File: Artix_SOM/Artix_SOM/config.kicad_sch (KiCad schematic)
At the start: 9 parts, among them SW1 SW_Push, U1 XC7A100T-FGG676

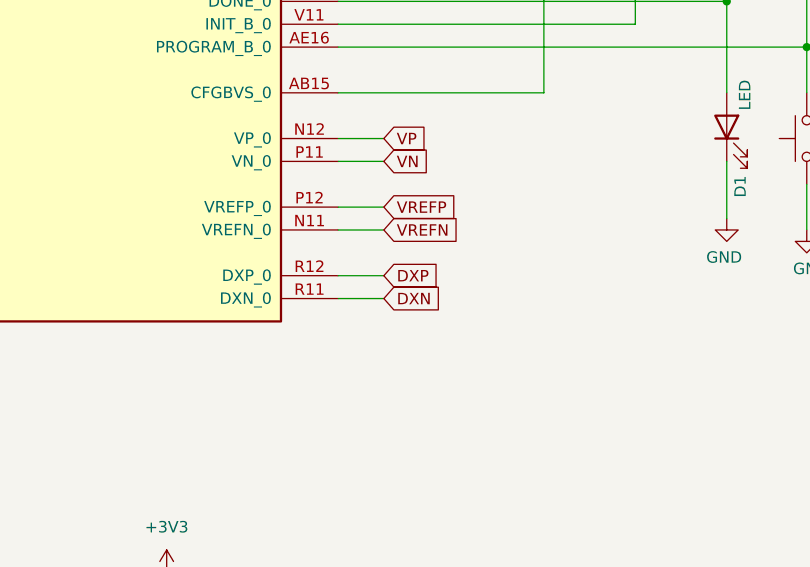
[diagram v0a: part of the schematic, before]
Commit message: update
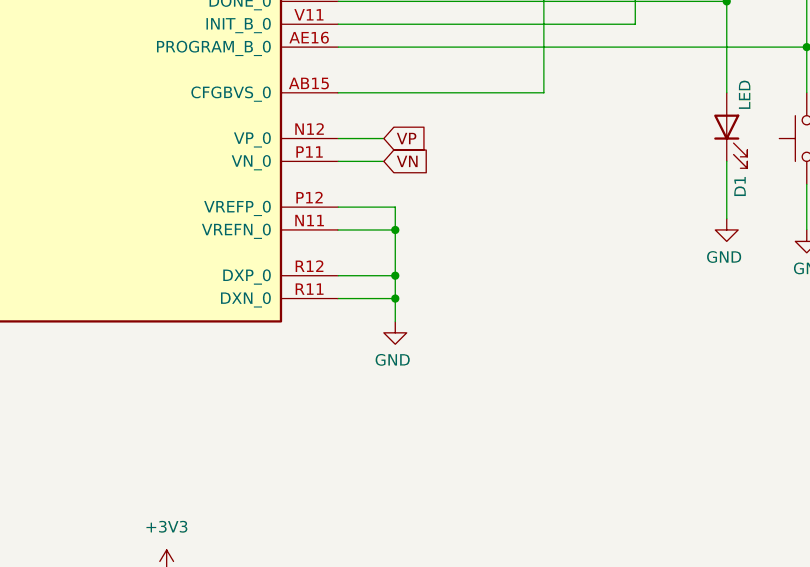
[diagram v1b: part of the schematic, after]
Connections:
- net DXN is gone; now on net GND: U1.R11 (DXN_0)
- net DXP is gone; now on net GND: U1.R12 (DXP_0)
- net VREFN is gone; now on net GND: U1.N11 (VREFN_0)
- net VREFP is gone; now on net GND: U1.P12 (VREFP_0)
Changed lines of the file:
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@@
+	)
+	(junction
+		(at 160.02 139.7)
+		(diameter 0)
+		(color 0 0 0 0)
+	)
+	(junction
+		(at 160.02 142.24)
+		(diameter 0)
+		(color 0 0 0 0)
 	)
 	(junction
@@
 	)
 	(junction
+		(at 160.02 134.62)
+		(diameter 0)
+		(color 0 0 0 0)
+	)
+	(junction
 		(at 191.77 93.98)
 		(diameter 0)
@@
 	(wire
 		(pts
+			(xy 160.02 132.08) (xy 160.02 134.62)
+		)
+		(stroke
+			(width 0)
+			(type default)
+		)
+	)
+	(wire
+		(pts
 			(xy 153.67 124.46) (xy 158.75 124.46)
 		)
@@
 	(wire
 		(pts
-			(xy 153.67 134.62) (xy 158.75 134.62)
+			(xy 153.67 134.62) (xy 160.02 134.62)
 		)
 		(stroke
@@
 	(wire
 		(pts
-			(xy 153.67 142.24) (xy 158.75 142.24)
-		)
-		(stroke
-			(width 0)
-			(type default)
-		)
-	)
-	(wire
-		(pts
-			(xy 153.67 132.08) (xy 158.75 132.08)
+			(xy 153.67 132.08) (xy 160.02 132.08)
 		)
 		(stroke
@@
 	(wire
 		(pts
-			(xy 153.67 139.7) (xy 158.75 139.7)
-		)
-		(stroke
-			(width 0)
-			(type default)
-		)
-	)
-	(wire
-		(pts
 			(xy 153.67 109.22) (xy 196.85 109.22)
 		)
@@
 	(wire
 		(pts
+			(xy 153.67 139.7) (xy 160.02 139.7)
+		)
+		(stroke
+			(width 0)
+			(type default)
+		)
+	)
+	(wire
+		(pts
 			(xy 153.67 83.82) (xy 160.02 83.82)
 		)
@@
 	(wire
 		(pts
+			(xy 153.67 142.24) (xy 160.02 142.24)
+		)
+		(stroke
+			(width 0)
+			(type default)
+		)
+	)
+	(wire
+		(pts
 			(xy 134.62 186.69) (xy 128.27 186.69)
 		)
@@
 	(wire
 		(pts
+			(xy 160.02 139.7) (xy 160.02 142.24)
+		)
+		(stroke
+			(width 0)
+			(type default)
+		)
+	)
+	(wire
+		(pts
 			(xy 153.67 114.3) (xy 205.74 114.3)
 		)
@@
 	(wire
 		(pts
+			(xy 160.02 142.24) (xy 160.02 144.78)
+		)
+		(stroke
+			(width 0)
+			(type default)
+		)
+	)
+	(wire
+		(pts
 			(xy 153.67 88.9) (xy 160.02 88.9)
+		)
+		(stroke
+			(width 0)
+			(type default)
+		)
+	)
+	(wire
+		(pts
+			(xy 160.02 134.62) (xy 160.02 139.7)
 		)
 		(stroke
@@
 		)
 	)
-	(global_label "VREFN"
-		(shape input)
-		(at 158.75 134.62 0)
-		(fields_autoplaced yes)
-		(effects
-			(font
-				(size 1.27 1.27)
-			)
-			(justify left)
-		)
-		(property "Intersheetrefs" "${INTERSHEET_REFS}"
-			(at 167.6619 134.62 0)
-			(effects
-				(font
-					(size 1.27 1.27)
-				)
-				(justify left)
-				(hide yes)
-			)
-		)
-	)
 	(global_label "VP"
 		(shape input)
@@
 					(size 1.27 1.27)
 				)
-				(hide yes)
-			)
-		)
-	)
-	(global_label "DXN"
-		(shape input)
-		(at 158.75 142.24 0)
-		(fields_autoplaced yes)
-		(effects
-			(font
-				(size 1.27 1.27)
-			)
-			(justify left)
-		)
-		(property "Intersheetrefs" "${INTERSHEET_REFS}"
-			(at 165.5452 142.24 0)
-			(effects
-				(font
-					(size 1.27 1.27)
-				)
-				(justify left)
-				(hide yes)
-			)
-		)
-	)
-	(global_label "DXP"
-		(shape input)
-		(at 158.75 139.7 0)
-		(fields_autoplaced yes)
-		(effects
-			(font
-				(size 1.27 1.27)
-			)
-			(justify left)
-		)
-		(property "Intersheetrefs" "${INTERSHEET_REFS}"
-			(at 165.4847 139.7 0)
-			(effects
-				(font
-					(size 1.27 1.27)
-				)
-				(justify left)
-				(hide yes)
-			)
-		)
-	)
-	(global_label "VREFP"
-		(shape input)
-		(at 158.75 132.08 0)
-		(fields_autoplaced yes)
-		(effects
-			(font
-				(size 1.27 1.27)
-			)
-			(justify left)
-		)
-		(property "Intersheetrefs" "${INTERSHEET_REFS}"
-			(at 167.6014 132.08 0)
-			(effects
-				(font
-					(size 1.27 1.27)
-				)
-				(justify left)
 				(hide yes)
 			)
@@
 					(unit 1)
 				)
+			)
+		)
+	)
+	(symbol
+		(lib_id "power:GND")
+		(at 160.02 144.78 0)
+		(unit 1)
+		(exclude_from_sim no)
+		(in_bom yes)
+		(on_board yes)
+		(dnp no)
+		(property "Reference" "#PWR097"
+			(at 160.02 151.13 0)
+			(effects
+				(font
+					(size 1.27 1.27)
+				)
+				(hide yes)
+			)
+		)
+		(property "Value" "GND"
+			(at 157.734 149.098 0)
+			(effects
+				(font
+					(size 1.27 1.27)
+				)
+				(justify left)
+			)
+		)
+		(property "Footprint" ""
+			(at 160.02 144.78 0)
+			(effects
+				(font
+					(size 1.27 1.27)
+				)
+				(hide yes)
+			)
+		)
+		(property "Datasheet" ""
+			(at 160.02 144.78 0)
+			(effects
+				(font
+					(size 1.27 1.27)
+				)
+				(hide yes)
+			)
+		)
+		(property "Description" "Power symbol creates a global label with name \"GND\" , ground"
+			(at 160.02 144.78 0)
+			(effects
+				(font
+					(size 1.27 1.27)
+				)
+				(hide yes)
+			)
+		)
+		(pin "1"
+		)
+		(instances
+			(project "Artix_SOM"
+				(path "/c2221598-f078-4310-82f6-aed2a006194d/916a1e8f-bf41-4c79-9025-473ebee52cc2"
+					(reference "#PWR097")
+					(unit 1)
+				)

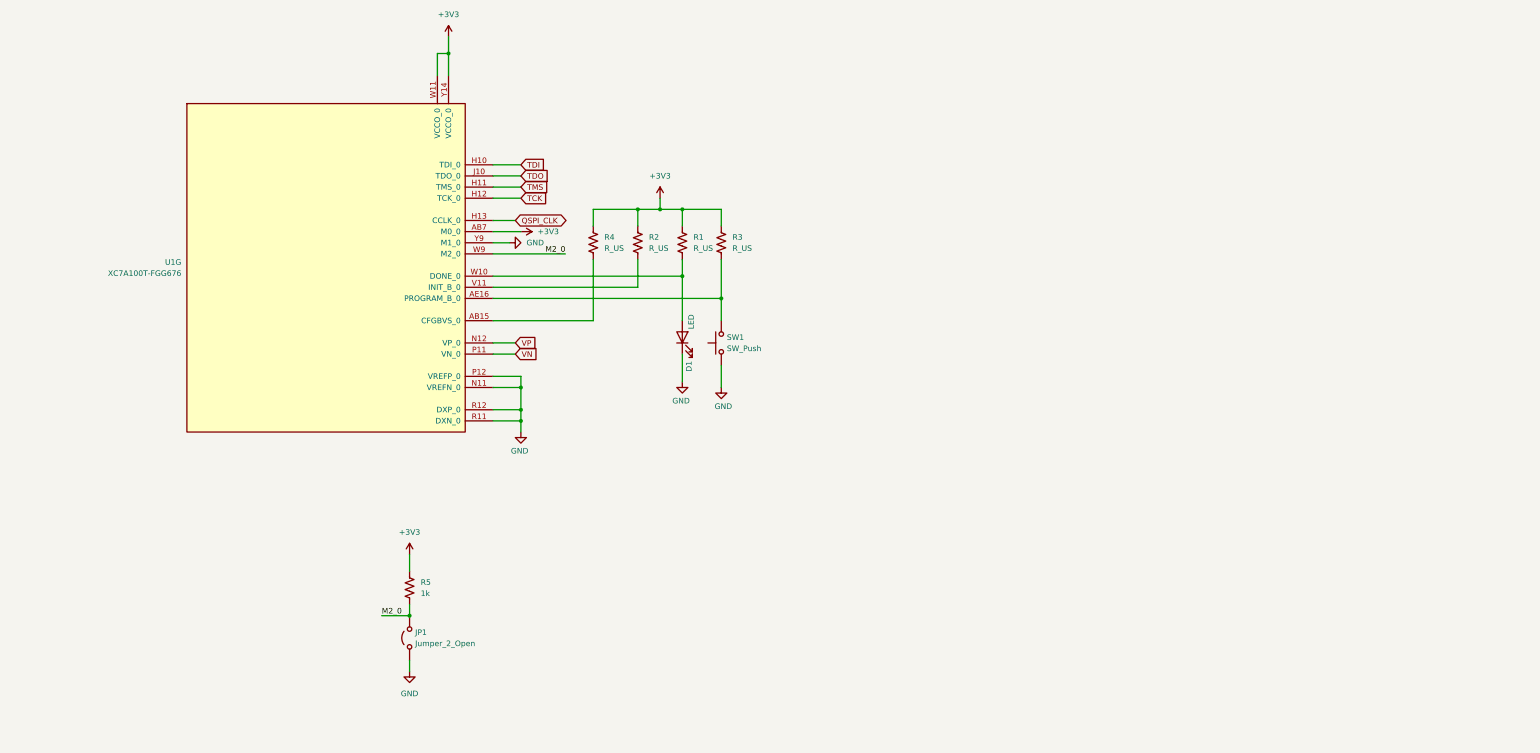
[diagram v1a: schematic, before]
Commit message: update
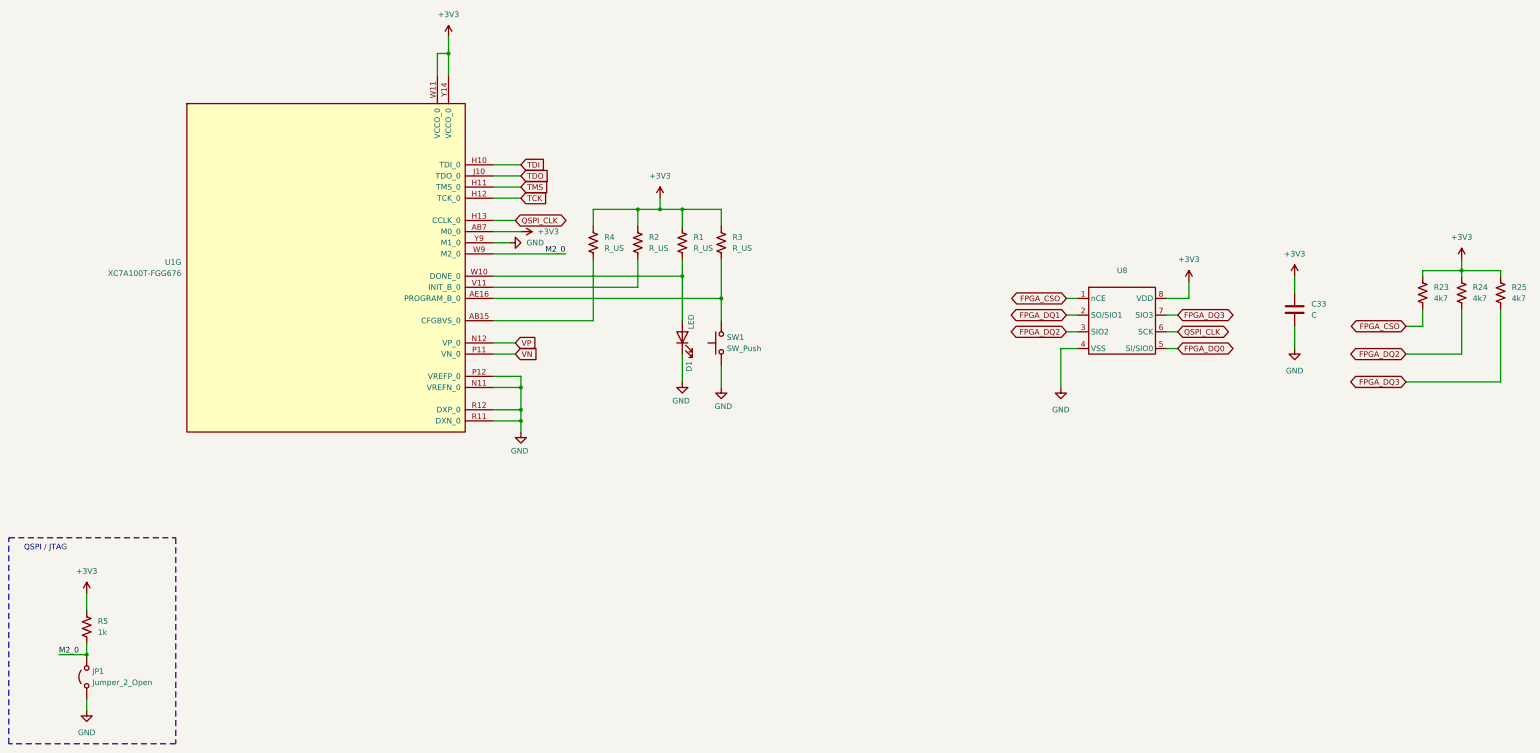
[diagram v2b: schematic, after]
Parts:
- added C33: C, symbol Device:C
- added R23, R24, R25: 4k7, symbol Device:R_US
- added U8: ~, symbol Sources:MT25QL128
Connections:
- net +3V3: now also C33.1, R23.1, R24.1, R25.1, U8.8 (VDD)
- net GND: now also C33.2, U8.4 (VSS)
- net QSPI_CLK: now also U8.6 (SCK)
- new net FPGA_CSO: R23.2, U8.1 (nCE)
- new net FPGA_DQ0: U8.5 (SI/SIO0)
- new net FPGA_DQ1: U8.2 (SO/SIO1)
- new net FPGA_DQ2: R24.2, U8.3 (SIO2)
- new net FPGA_DQ3: R25.2, U8.7 (SIO3)
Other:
- note added: "QSPI / JTAG"
- moved on the sheet: JP1, R5
